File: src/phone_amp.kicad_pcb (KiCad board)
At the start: 2 copper layers, 11.6 x 56.1 mm, 41 parts, among them J1 M_USB_B, J2 PJ313D, J3 PJ313D, J4 RJ9_4P4C, J5 RJ9_4P4C, SW1 SWITCH_INV, U1 TPA6139A2, U2 MCP6024, U3 TC1017

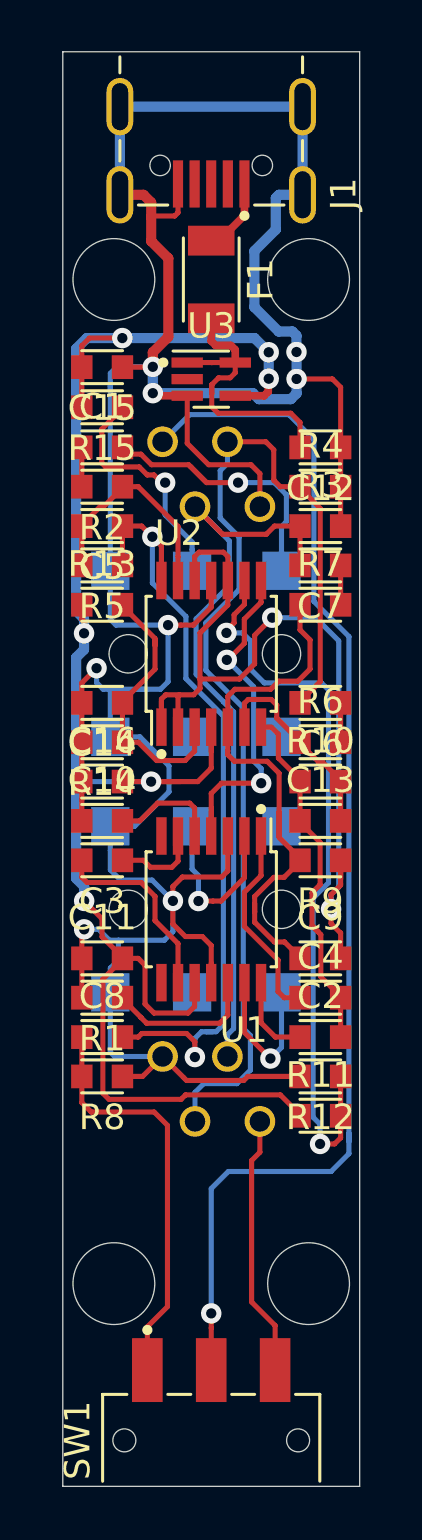
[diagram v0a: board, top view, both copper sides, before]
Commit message: Uploaded finished design.
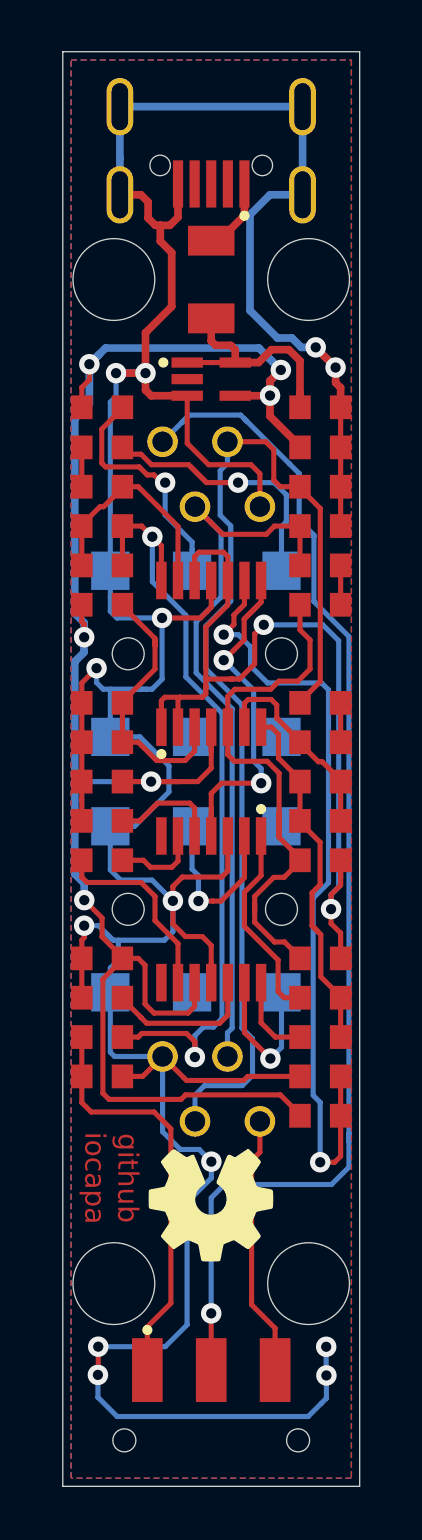
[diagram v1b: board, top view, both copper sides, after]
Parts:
- added G***: LOGO, footprints:OSH_LOGO, F.Cu at (139.7, 124.5)
- C1, C10, C11, C12, C13, C14, C15, C16, C2, C3, C4, C5, C6, C7, C8, C9, R1, R10, R11, R12, R13, R14, R15, R2, R3, R4, R5, R6, R7, R8, R9: footprint footprints:CHIP-0603 -> footprints:CHIP-0603-NO-SILK
- F1: footprint footprints:FUSE-1206 -> footprints:FUSE-1206-NO-SILK
- J1: footprint footprints:USB-MICRO-TH -> footprints:USB-MICRO-TH-NO-SILK
- J2, J3: footprint footprints:JACK-3.5MM -> footprints:JACK-3.5MM-NO-SILK
- J4, J5: footprint footprints:RJ9-4P4C -> footprints:RJ9-4P4C-NO-SILK
- SW1: footprint footprints:SWITCH-SPDT -> footprints:SWITCH-SPDT-NO-SILK
- U1, U2: footprint footprints:TSSOP-14 -> footprints:TSSOP-14-NO-SILK
- U3: footprint footprints:SC-70 -> footprints:SC-70-NO-SILK
- moved C15 9.10 mm to (144.0, 94.9)
- moved C12 1.57 mm to (144.0, 93.3)
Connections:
- J1 pad 2: (no net) -> Net-(J1-Pad2)
- J1 pad 3: (no net) -> Net-(J1-Pad3)
- J1 pad 4: (no net) -> Net-(J1-Pad4)
- J2 pad 1: (no net) -> Net-(J2-Pad1)
- J2 pad 2: (no net) -> Net-(J2-Pad2)
- J3 pad 2: (no net) -> Net-(J3-Pad2)
- J3 pad 6: (no net) -> Net-(J3-Pad6)
- U1 pad 7: (no net) -> Net-(U1-Pad7)
- U1 pad 8: (no net) -> Net-(U1-Pad8)
- U3 pad 2: (no net) -> Net-(U3-Pad2)
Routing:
- net GND: track 132.1 -> 155.1 mm, vias 8 -> 13
- net HS_SPK_P: track 32.0 -> 29.2 mm
- net Net-(C12-Pad2): track 12.2 -> 9.50 mm
- net +3V3: track 70.9 -> 73.3 mm
- net Net-(R11-Pad2): track 29.4 -> 30.8 mm
- net HP_MUTE: track 13.8 -> 14.7 mm
- net PHONE_MIC_P: track 48.7 -> 47.9 mm
- added copper zone on B.Cu, net GND
- added copper zone on F.Cu, net GND
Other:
- board text added: "github iocapa"
